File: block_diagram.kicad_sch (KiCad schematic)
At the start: 0 parts

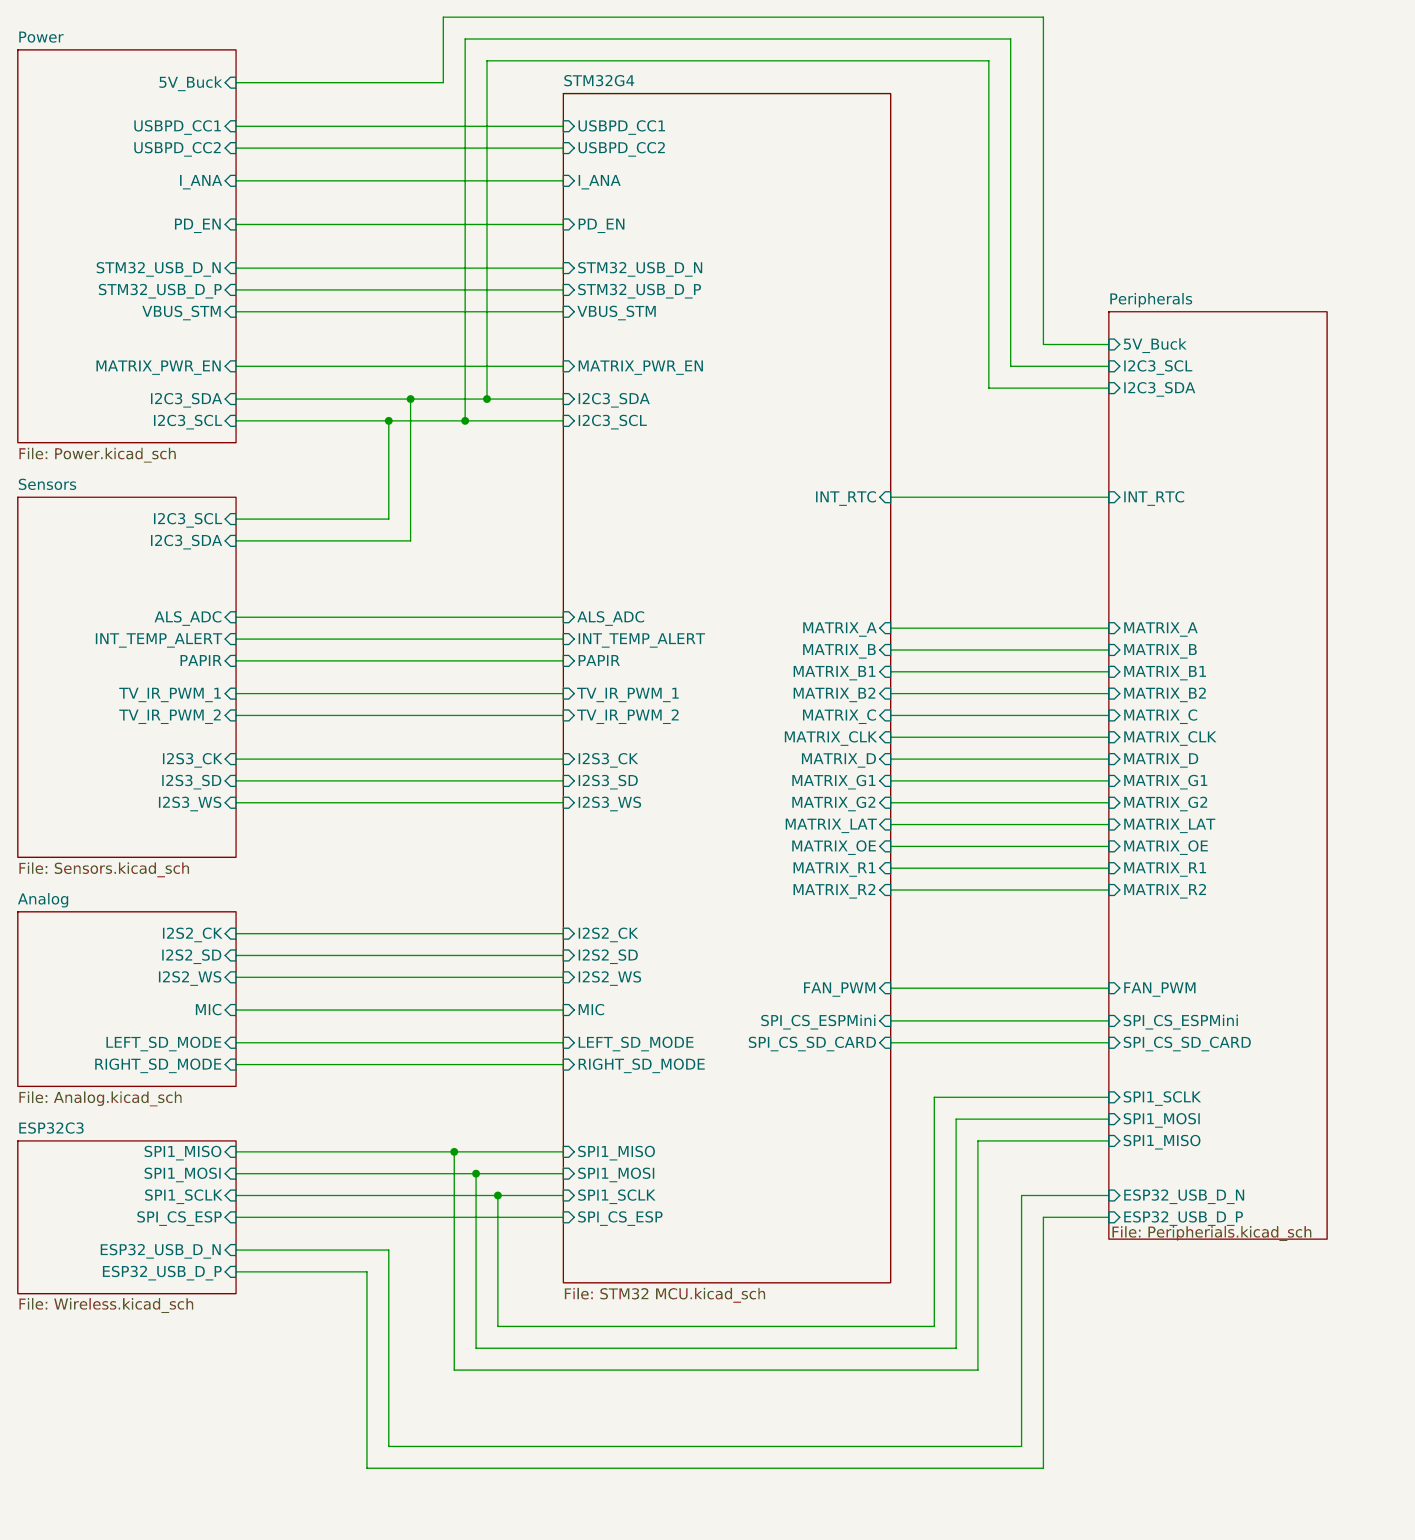
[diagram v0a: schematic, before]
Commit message: Fixed
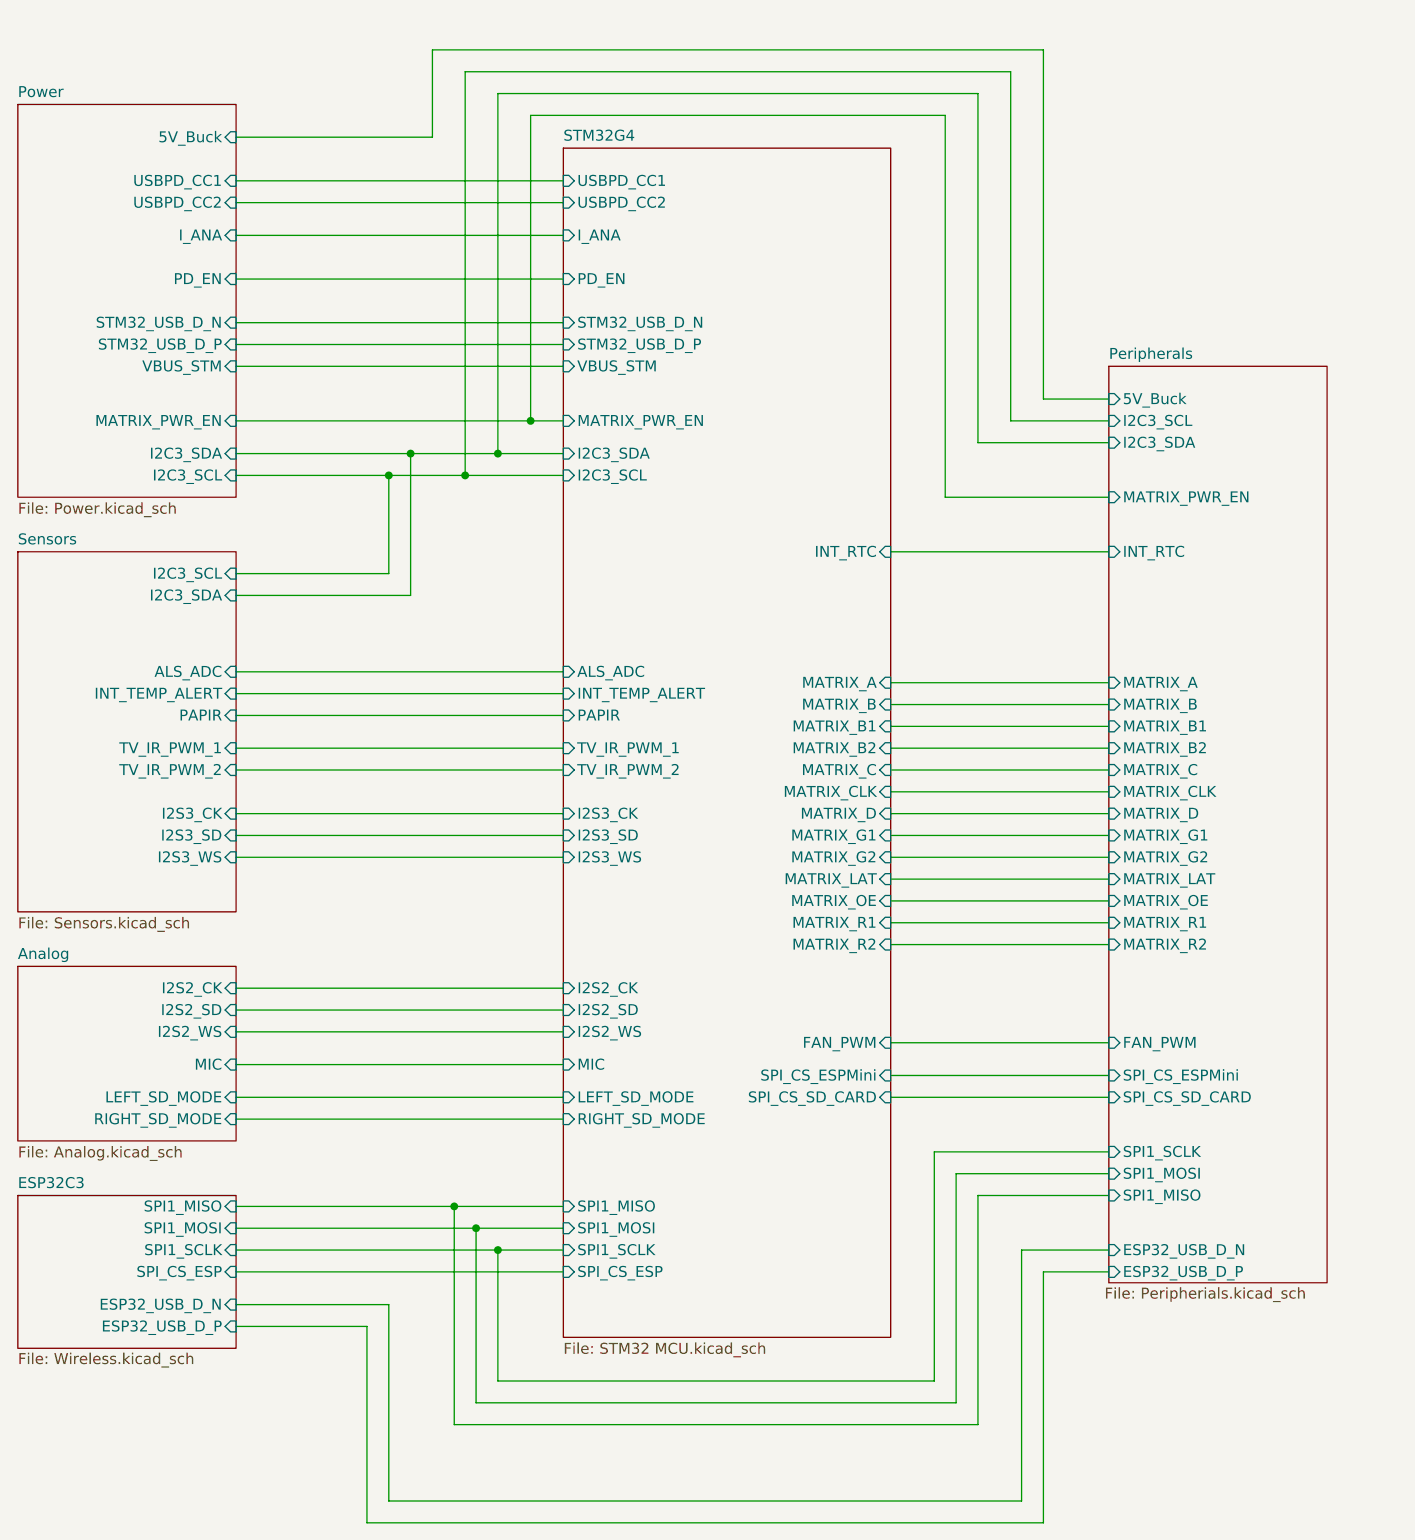
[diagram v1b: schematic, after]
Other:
- sheet Peripherals ports: added MATRIX_PWR_EN; removed none
